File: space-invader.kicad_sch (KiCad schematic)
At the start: 35 parts, among them SW1 SW_Push, SW10 SW_Push, SW11 SW_Push, SW12 SW_Push, SW13 SW_Push, SW14 SW_Push, SW15 SW_Push, SW16 SW_Push, SW17 SW_Push, SW2 SW_Push, SW3 SW_Push, SW4 SW_Push, SW5 SW_Push, SW6 SW_Push, SW7 SW_Push, SW8 SW_Push, SW9 SW_Push, U1 Seeeduino Xiao nRF52840

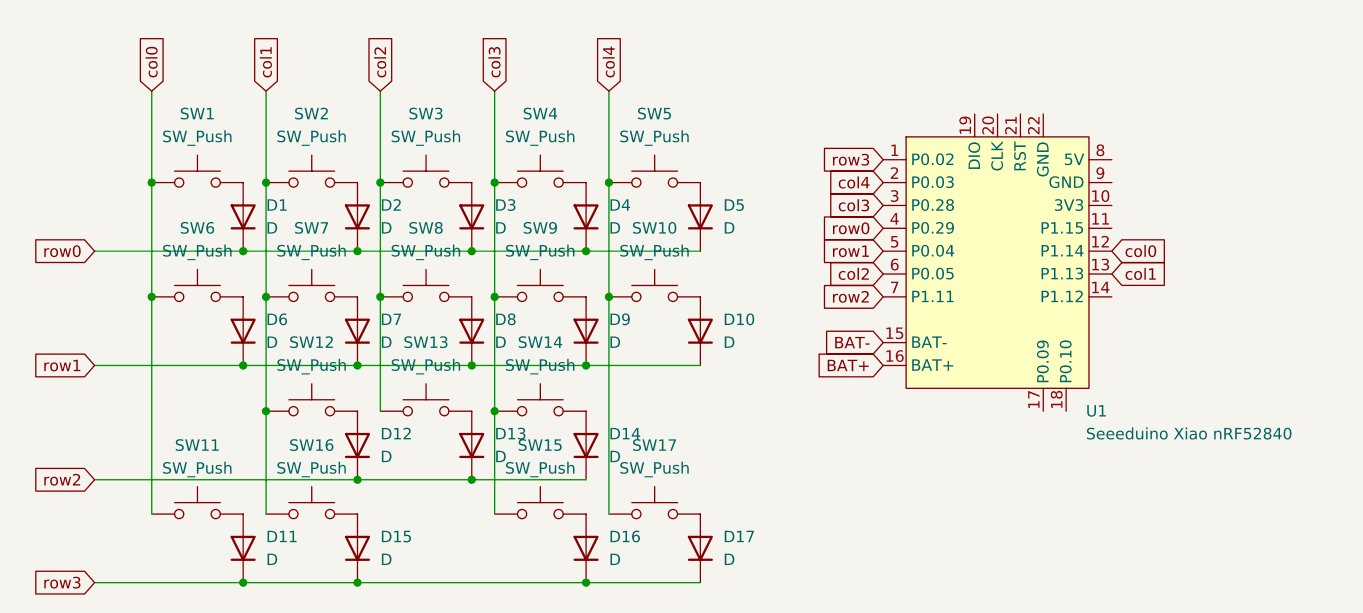
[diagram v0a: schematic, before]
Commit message: there be graphics
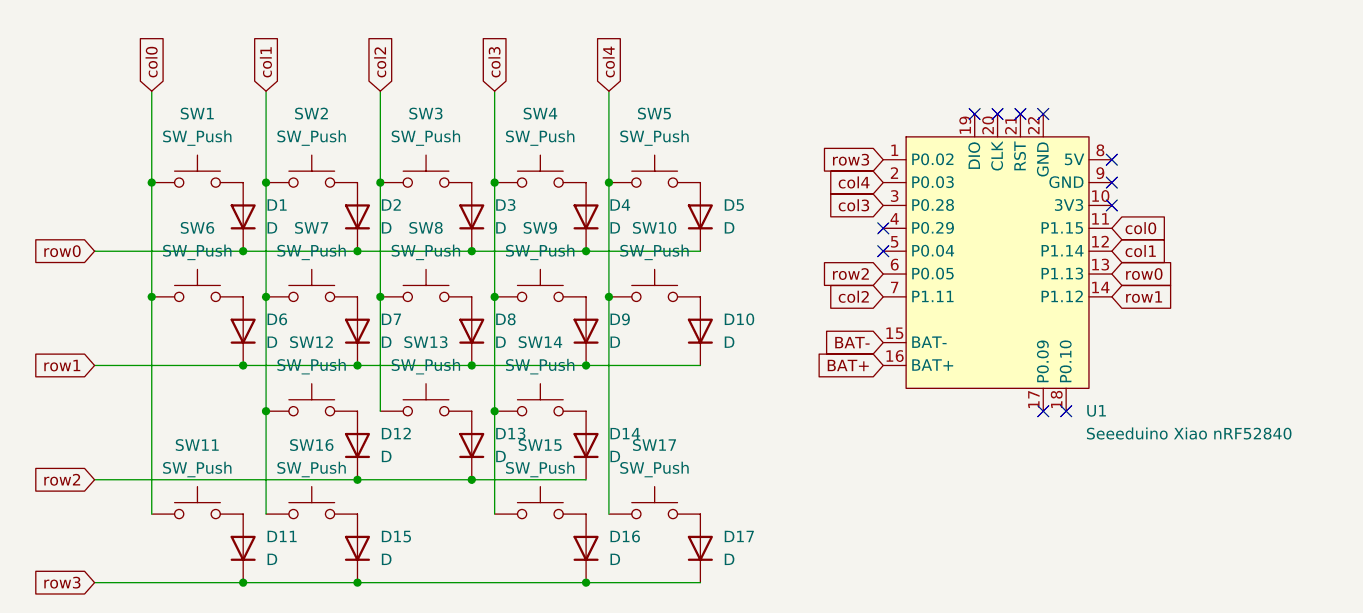
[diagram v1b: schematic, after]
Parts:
- U1: footprint PCM_marbastlib-xp-promicroish:Xiao_nRF52840_ACH -> PCM_marbastlib-xp-promicroish:Xiao_nRF52840_AC_Reflow
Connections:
- net col0: now also U1.11 (P1.15); no longer U1.12 (P1.14)
- net col1: now also U1.12 (P1.14); no longer U1.13 (P1.13)
- net col2: now also U1.7 (P1.11); no longer U1.6 (P0.05)
- net row0: now also U1.13 (P1.13); no longer U1.4 (P0.29)
- net row1: now also U1.14 (P1.12); no longer U1.5 (P0.04)
- net row2: now also U1.6 (P0.05); no longer U1.7 (P1.11)
- no-connect marks 0 -> 11
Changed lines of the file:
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@@
 		(color 0 0 0 0)
 	)
+	(no_connect
+		(at 138.43 24.13)
+	)
+	(no_connect
+		(at 140.97 57.15)
+	)
+	(no_connect
+		(at 130.81 24.13)
+	)
+	(no_connect
+		(at 138.43 57.15)
+	)
+	(no_connect
+		(at 133.35 24.13)
+	)
+	(no_connect
+		(at 120.65 39.37)
+	)
+	(no_connect
+		(at 135.89 24.13)
+	)
+	(no_connect
+		(at 120.65 36.83)
+	)
+	(no_connect
+		(at 146.05 34.29)
+	)
+	(no_connect
+		(at 146.05 29.21)
+	)
+	(no_connect
+		(at 146.05 31.75)
+	)
 	(wire
 		(pts
@@
 	(global_label "col1"
 		(shape input)
+		(at 146.05 39.37 0)
+		(fields_autoplaced yes)
+		(effects
+			(font
+				(size 1.27 1.27)
+			)
+			(justify left)
+		)
+		(property "Intersheetrefs" "${INTERSHEET_REFS}"
+			(at 153.1475 39.37 0)
+			(effects
+				(font
+					(size 1.27 1.27)
+				)
+				(justify left)
+				(hide yes)
+			)
+		)
+	)
+	(global_label "col0"
+		(shape input)
+		(at 146.05 36.83 0)
+		(fields_autoplaced yes)
+		(effects
+			(font
+				(size 1.27 1.27)
+			)
+			(justify left)
+		)
+		(property "Intersheetrefs" "${INTERSHEET_REFS}"
+			(at 153.1475 36.83 0)
+			(effects
+				(font
+					(size 1.27 1.27)
+				)
+				(justify left)
+				(hide yes)
+			)
+		)
+	)
+	(global_label "row0"
+		(shape input)
 		(at 146.05 41.91 0)
 		(fields_autoplaced yes)
@@
 		)
 		(property "Intersheetrefs" "${INTERSHEET_REFS}"
-			(at 153.1475 41.91 0)
+			(at 153.5104 41.91 0)
 			(effects
 				(font
@@
 		)
 	)
-	(global_label "col0"
-		(shape input)
-		(at 146.05 39.37 0)
+	(global_label "col4"
+		(shape input)
+		(at 90.17 21.59 90)
 		(fields_autoplaced yes)
 		(effects
@@
 		)
 		(property "Intersheetrefs" "${INTERSHEET_REFS}"
-			(at 153.1475 39.37 0)
+			(at 90.17 14.4925 90)
 			(effects
 				(font
@@
 		)
 	)
-	(global_label "row0"
-		(shape input)
-		(at 120.65 36.83 180)
+	(global_label "row2"
+		(shape input)
+		(at 120.65 41.91 180)
 		(fields_autoplaced yes)
 		(effects
@@
 		)
 		(property "Intersheetrefs" "${INTERSHEET_REFS}"
-			(at 113.1896 36.83 0)
+			(at 113.1896 41.91 0)
+			(effects
+				(font
+					(size 1.27 1.27)
+				)
+				(justify right)
+				(hide yes)
+			)
+		)
+	)
+	(global_label "row1"
+		(shape input)
+		(at 146.05 44.45 0)
+		(fields_autoplaced yes)
+		(effects
+			(font
+				(size 1.27 1.27)
+			)
+			(justify left)
+		)
+		(property "Intersheetrefs" "${INTERSHEET_REFS}"
+			(at 153.5104 44.45 0)
+			(effects
+				(font
+					(size 1.27 1.27)
+				)
+				(justify left)
+				(hide yes)
+			)
+		)
+	)
+	(global_label "row1"
+		(shape input)
+		(at 33.02 52.07 180)
+		(fields_autoplaced yes)
+		(effects
+			(font
+				(size 1.27 1.27)
+			)
+			(justify right)
+		)
+		(property "Intersheetrefs" "${INTERSHEET_REFS}"
+			(at 25.5596 52.07 0)
 			(effects
 				(font
@@
 	(global_label "col4"
 		(shape input)
-		(at 90.17 21.59 90)
-		(fields_autoplaced yes)
-		(effects
-			(font
-				(size 1.27 1.27)
-			)
-			(justify left)
-		)
-		(property "Intersheetrefs" "${INTERSHEET_REFS}"
-			(at 90.17 14.4925 90)
-			(effects
-				(font
-					(size 1.27 1.27)
-				)
-				(justify left)
-				(hide yes)
-			)
-		)
-	)
-	(global_label "row2"
+		(at 120.65 31.75 180)
+		(fields_autoplaced yes)
+		(effects
+			(font
+				(size 1.27 1.27)
+			)
+			(justify right)
+		)
+		(property "Intersheetrefs" "${INTERSHEET_REFS}"
+			(at 113.5525 31.75 0)
+			(effects
+				(font
+					(size 1.27 1.27)
+				)
+				(justify right)
+				(hide yes)
+			)
+		)
+	)
+	(global_label "col2"
 		(shape input)
 		(at 120.65 44.45 180)
@@
 		)
 		(property "Intersheetrefs" "${INTERSHEET_REFS}"
-			(at 113.1896 44.45 0)
-			(effects
-				(font
-					(size 1.27 1.27)
-				)
-				(justify right)
-				(hide yes)
-			)
-		)
-	)
-	(global_label "row1"
-		(shape input)
-		(at 120.65 39.37 180)
-		(fields_autoplaced yes)
-		(effects
-			(font
-				(size 1.27 1.27)
-			)
-			(justify right)
-		)
-		(property "Intersheetrefs" "${INTERSHEET_REFS}"
-			(at 113.1896 39.37 0)
-			(effects
-				(font
-					(size 1.27 1.27)
-				)
-				(justify right)
-				(hide yes)
-			)
-		)
-	)
-	(global_label "row1"
-		(shape input)
-		(at 33.02 52.07 180)
-		(fields_autoplaced yes)
-		(effects
-			(font
-				(size 1.27 1.27)
-			)
-			(justify right)
-		)
-		(property "Intersheetrefs" "${INTERSHEET_REFS}"
-			(at 25.5596 52.07 0)
-			(effects
-				(font
-					(size 1.27 1.27)
-				)
-				(justify right)
-				(hide yes)
-			)
-		)
-	)
-	(global_label "col4"
-		(shape input)
-		(at 120.65 31.75 180)
-		(fields_autoplaced yes)
-		(effects
-			(font
-				(size 1.27 1.27)
-			)
-			(justify right)
-		)
-		(property "Intersheetrefs" "${INTERSHEET_REFS}"
-			(at 113.5525 31.75 0)
-			(effects
-				(font
-					(size 1.27 1.27)
-				)
-				(justify right)
-				(hide yes)
-			)
-		)
-	)
-	(global_label "col2"
-		(shape input)
-		(at 120.65 41.91 180)
-		(fields_autoplaced yes)
-		(effects
-			(font
-				(size 1.27 1.27)
-			)
-			(justify right)
-		)
-		(property "Intersheetrefs" "${INTERSHEET_REFS}"
-			(at 113.5525 41.91 0)
+			(at 113.5525 44.45 0)
 			(effects
 				(font
@@
 			)
 		)
-		(property "Footprint" "PCM_marbastlib-xp-promicroish:Xiao_nRF52840_ACH"
+		(property "Footprint" "PCM_marbastlib-xp-promicroish:Xiao_nRF52840_AC_Reflow"
 			(at 133.35 73.66 0)
 			(effects
